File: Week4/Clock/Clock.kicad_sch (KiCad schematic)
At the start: 46 parts, among them J1 Power_inlet_vertical, J2 Conn_01x06, SW1 RotaryEncoder_Switch, SW2 Omron_B3F_SPST, U2 ATmega328-PU, U3 L7805_TO92, U4 DS1307_DIP-8, U5 MAX7219, U6 MAX7219, Y1 Crystal 16MHZ, Y2 Crystal_32768Hz

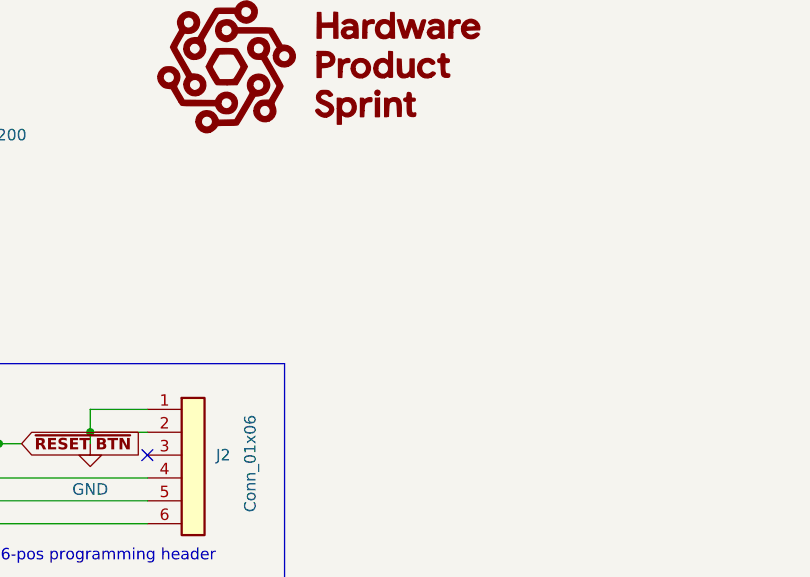
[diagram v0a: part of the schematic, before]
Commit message: Added Fetus Arduino Code
Baby Clock Code has been added
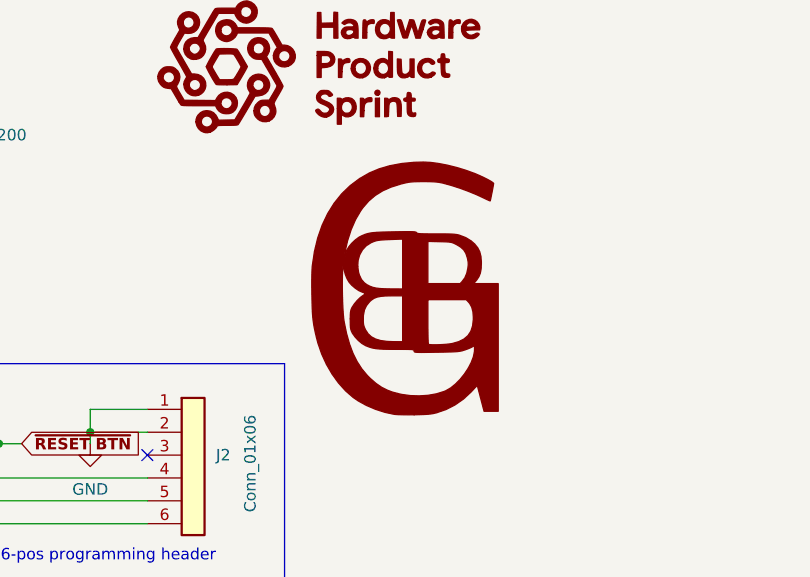
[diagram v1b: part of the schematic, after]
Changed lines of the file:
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@@
     (pin "2")
+  )
+  (symbol (lib_id "Logo:LOGO") (at 245.11 58.42 0) (unit 1)
+    (in_bom yes) (on_board yes) (fields_autoplaced)
+    (property "Reference" "#G2" (id 0) (at 245.11 37.8175 0)
+      (effects (font (size 1.27 1.27)) hide)
+    )
+    (property "Value" "LOGO" (id 1) (at 245.11 79.0225 0)
+      (effects (font (size 1.27 1.27)) hide)
+    )
+    (property "Footprint" "" (id 2) (at 245.11 58.42 0)
+      (effects (font (size 1.27 1.27)) hide)
+    )
+    (property "Datasheet" "" (id 3) (at 245.11 58.42 0)
+      (effects (font (size 1.27 1.27)) hide)
+    )
   )
   (symbol (lib_id "HPS:VCC") (at 57.15 83.82 0) (unit 1)
@@
       (reference "#G1") (unit 1) (value "HPS_Logo") (footprint "")
     )
+    (path "/f46ac623-4ddf-4dd9-909e-dde17c33c099"
+      (reference "#G2") (unit 1) (value "LOGO") (footprint "")
+    )
     (path "/fb4d5b8c-776c-40ea-804f-0ca9c5d8e8fe"
